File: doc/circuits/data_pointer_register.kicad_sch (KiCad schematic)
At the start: 8 parts, among them U1 74LS193, U2 74LS193, U3 74LS245, U4 74LS04, U5 74LS193, U6 74LS193, U7 74LS32, U9 74LS245

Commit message: documented data and datapointer registers
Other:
- company: (none) -> J. Heit

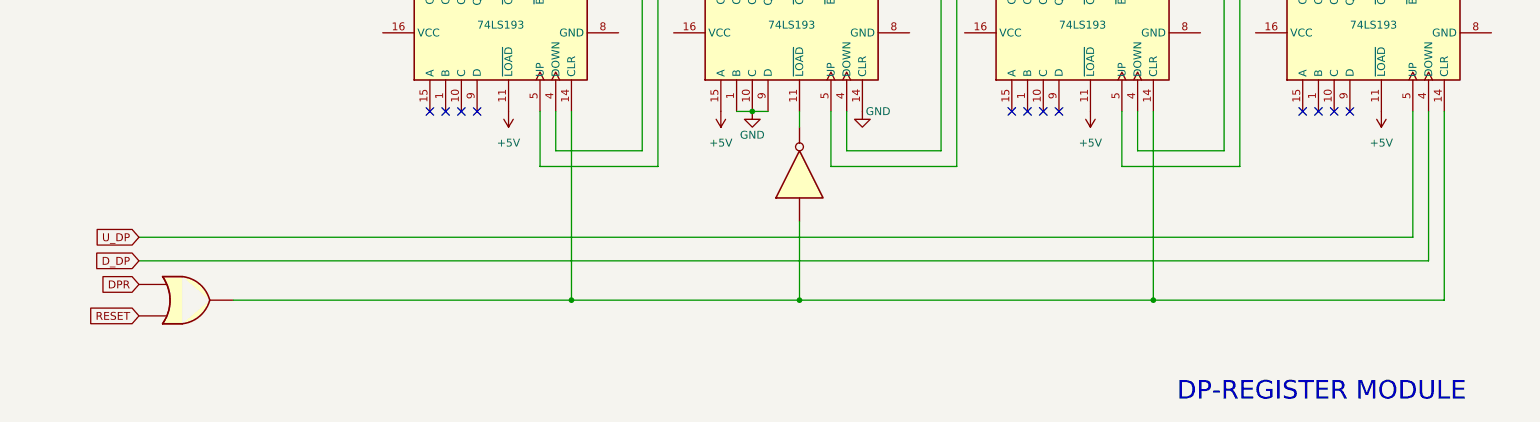
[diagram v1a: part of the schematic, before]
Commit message: more documentation
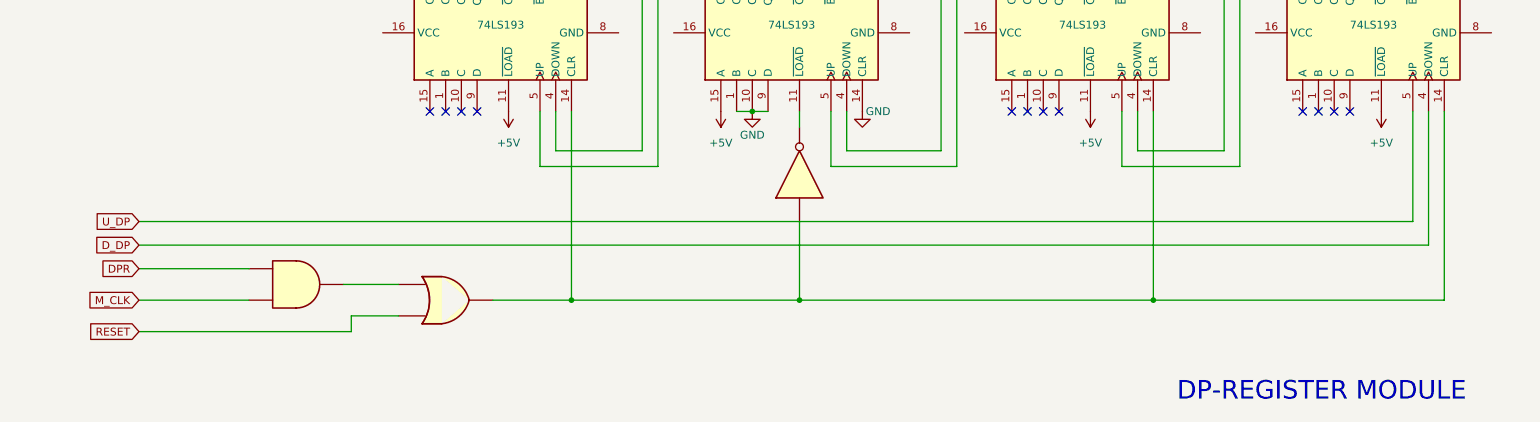
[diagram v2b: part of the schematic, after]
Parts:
- added U8: 74LS08, symbol 74xx:74LS08
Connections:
- net DPR: now also U8.1; no longer U7.1
- new net: U7.1, U8.3
- new net M_CLK: U8.2
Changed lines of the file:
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@@
+	)
+	(junction
+		(at 135.89 129.54)
+		(diameter 0)
+		(color 0 0 0 0)
 	)
 	(junction
@@
 	)
 	(junction
-		(at 106.68 160.02)
-		(diameter 0)
-		(color 0 0 0 0)
-	)
-	(junction
 		(at 200.66 160.02)
-		(diameter 0)
-		(color 0 0 0 0)
-	)
-	(junction
-		(at 135.89 129.54)
 		(diameter 0)
 		(color 0 0 0 0)
@@
 		(color 0 0 0 0)
 	)
+	(junction
+		(at 106.68 160.02)
+		(diameter 0)
+		(color 0 0 0 0)
+	)
 	(no_connect
 		(at 91.44 129.54)
@@
 	(wire
 		(pts
-			(xy 36.83 149.86) (xy 242.57 149.86)
+			(xy 36.83 147.32) (xy 242.57 147.32)
+		)
+		(stroke
+			(width 0)
+			(type default)
+		)
+	)
+	(wire
+		(pts
+			(xy 71.12 165.1) (xy 71.12 162.56)
 		)
 		(stroke
@@
 	(wire
 		(pts
+			(xy 143.51 147.32) (xy 143.51 160.02)
+		)
+		(stroke
+			(width 0)
+			(type default)
+		)
+	)
+	(wire
+		(pts
 			(xy 88.9 33.02) (xy 88.9 40.64)
 		)
@@
 	(wire
 		(pts
-			(xy 52.07 160.02) (xy 106.68 160.02)
+			(xy 93.98 160.02) (xy 106.68 160.02)
 		)
 		(stroke
@@
 	(wire
 		(pts
-			(xy 242.57 149.86) (xy 242.57 129.54)
+			(xy 242.57 147.32) (xy 242.57 129.54)
 		)
 		(stroke
@@
 	(wire
 		(pts
+			(xy 36.83 154.94) (xy 54.61 154.94)
+		)
+		(stroke
+			(width 0)
+			(type default)
+		)
+	)
+	(wire
+		(pts
 			(xy 120.65 100.33) (xy 120.65 138.43)
 		)
@@
 		)
 	)
+	(wire
+		(pts
+			(xy 36.83 165.1) (xy 71.12 165.1)
+		)
+		(stroke
+			(width 0)
+			(type default)
+		)
+	)
 	(bus
 		(pts
@@
 	(wire
 		(pts
-			(xy 143.51 147.32) (xy 143.51 160.02)
-		)
-		(stroke
-			(width 0)
-			(type default)
-		)
-	)
-	(wire
-		(pts
 			(xy 182.88 38.1) (xy 182.88 40.64)
 		)
@@
 	(wire
 		(pts
-			(xy 36.83 153.67) (xy 245.11 153.67)
+			(xy 36.83 151.13) (xy 245.11 151.13)
 		)
 		(stroke
@@
 	(wire
 		(pts
+			(xy 69.85 157.48) (xy 78.74 157.48)
+		)
+		(stroke
+			(width 0)
+			(type default)
+		)
+	)
+	(wire
+		(pts
 			(xy 177.8 38.1) (xy 177.8 40.64)
 		)
@@
 	(wire
 		(pts
+			(xy 36.83 160.02) (xy 54.61 160.02)
+		)
+		(stroke
+			(width 0)
+			(type default)
+		)
+	)
+	(wire
+		(pts
 			(xy 177.8 66.04) (xy 177.8 104.14)
 		)
@@
 	(wire
 		(pts
-			(xy 245.11 153.67) (xy 245.11 129.54)
+			(xy 245.11 151.13) (xy 245.11 129.54)
 		)
 		(stroke
@@
 		(pts
 			(xy 96.52 33.02) (xy 96.52 40.64)
+		)
+		(stroke
+			(width 0)
+			(type default)
+		)
+	)
+	(wire
+		(pts
+			(xy 71.12 162.56) (xy 78.74 162.56)
 		)
 		(stroke
@@
 	(global_label "DPR"
 		(shape input)
-		(at 36.83 157.48 180)
+		(at 36.83 154.94 180)
 		(fields_autoplaced yes)
 		(effects
@@
 		)
 		(property "Intersheetrefs" "${INTERSHEET_REFS}"
-			(at 30.0348 157.48 0)
+			(at 30.0348 154.94 0)
 			(effects
 				(font
@@
 	(global_label "U_DP"
 		(shape input)
-		(at 36.83 149.86 180)
+		(at 36.83 147.32 180)
 		(fields_autoplaced yes)
 		(effects
@@
 		)
 		(property "Intersheetrefs" "${INTERSHEET_REFS}"
-			(at 29.0067 149.86 0)
+			(at 29.0067 147.32 0)
 			(effects
 				(font
@@
 	(global_label "RESET"
 		(shape input)
-		(at 36.83 162.56 180)
+		(at 36.83 165.1 180)
 		(fields_autoplaced yes)
 		(effects
@@
 		)
 		(property "Intersheetrefs" "${INTERSHEET_REFS}"
-			(at 28.0997 162.56 0)
+			(at 28.0997 165.1 0)
 			(effects
 				(font
@@
 	(global_label "D_DP"
 		(shape input)
-		(at 36.83 153.67 180)
+		(at 36.83 151.13 180)
 		(fields_autoplaced yes)
 		(effects
@@
 		)
 		(property "Intersheetrefs" "${INTERSHEET_REFS}"
-			(at 29.0672 153.67 0)
+			(at 29.0672 151.13 0)
 			(effects
 				(font
@@
 		(property "Intersheetrefs" "${INTERSHEET_REFS}"
 			(at 18.9072 30.48 0)
+			(effects
+				(font
+					(size 1.27 1.27)
+				)
+				(justify right)
+				(hide yes)
+			)
+		)
+	)
+	(global_label "M_CLK"
+		(shape input)
+		(at 36.83 160.02 180)
+		(fields_autoplaced yes)
+		(effects
+			(font
+				(size 1.27 1.27)
+			)
+			(justify right)
+		)
+		(property "Intersheetrefs" "${INTERSHEET_REFS}"
+			(at 27.8577 160.02 0)
 			(effects
 				(font
@@
 	)
 	(symbol
+		(lib_id "74xx:74LS08")
+		(at 62.23 157.48 0)
+		(unit 1)
+		(exclude_from_sim no)
+		(in_bom yes)
+		(on_board yes)
+		(dnp no)
+		(fields_autoplaced yes)
+		(property "Reference" "U8"
+			(at 62.2217 148.59 0)
+			(effects
+				(font
+					(size 1.27 1.27)
+				)
+				(hide yes)
+			)
+		)
+		(property "Value" "74LS08"
+			(at 62.2217 151.13 0)
+			(effects
+				(font
+					(size 1.27 1.27)
+				)
+				(hide yes)
+			)
+		)
+		(property "Footprint" ""
+			(at 62.23 157.48 0)
+			(effects
+				(font
+					(size 1.27 1.27)
+				)
+				(hide yes)
+			)
+		)
+		(property "Datasheet" "http://www.ti.com/lit/gpn/sn74LS08"
+			(at 62.23 157.48 0)
+			(effects
+				(font
+					(size 1.27 1.27)
+				)
+				(hide yes)
+			)
+		)
+		(property "Description" "Quad And2"
+			(at 62.23 157.48 0)
+			(effects
+				(font
+					(size 1.27 1.27)
+				)
+				(hide yes)
+			)
+		)
+		(pin "4"
+		)
+		(pin "6"
+		)
+		(pin "8"
+		)
+		(pin "9"
+		)
+		(pin "14"
+		)
+		(pin "10"
+		)
+		(pin "2"
+		)
+		(pin "1"
+		)
+		(pin "11"
+		)
+		(pin "13"
+		)
+		(pin "5"
+		)
+		(pin "12"
+		)
+		(pin "7"
+		)
+		(pin "3"
+		)
+		(instances
+			(project ""
+				(path "/469d95a3-59b6-4996-9093-6de4f67dd984"
+					(reference "U8")
+					(unit 1)
+				)
+			)
+		)
+	)
+	(symbol
 		(lib_id "74xx:74LS193")
 		(at 234.95 116.84 90)
@@
 	(symbol
 		(lib_id "74xx:74LS32")
-		(at 44.45 160.02 0)
+		(at 86.36 160.02 0)
 		(unit 1)
 		(exclude_from_sim no)
@@
 		(fields_autoplaced yes)
 		(property "Reference" "U7"
-			(at 44.45 151.13 0)
+			(at 86.36 151.13 0)
 			(effects
 				(font
@@
 		)
 		(property "Value" "74LS32"
-			(at 44.45 153.67 0)
+			(at 86.36 153.67 0)
 			(effects
 				(font
@@
 		)
 		(property "Footprint" ""
-			(at 44.45 160.02 0)
+			(at 86.36 160.02 0)
 			(effects
 				(font
@@
 		)
 		(property "Datasheet" "http://www.ti.com/lit/gpn/sn74LS32"
-			(at 44.45 160.02 0)
+			(at 86.36 160.02 0)
 			(effects
 				(font
@@
 		)
 		(property "Description" ""
-			(at 44.45 160.02 0)
-			(effects
-				(font
+			(at 86.36 160.02 0)
+			(effects
+				(font
